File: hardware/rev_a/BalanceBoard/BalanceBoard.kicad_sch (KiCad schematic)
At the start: 49 parts, among them J1 47491-0001-TR425, J2 5103309-1, T00 TestPoints, T01 TestPoints, T02 TestPoints, T03 TestPoints, T04 TestPoints, T05 TestPoints, T06 TestPoints, T07 TestPoints, T10 TestPoints, T11 TestPoints, T12 TestPoints, T13 TestPoints, T14 TestPoints, T15 TestPoints, T16 TestPoints, T17 TestPoints, T21 TestPoints, T31 TestPoints, T32 TestPoints, T33 TestPoints, T40 TestPoints, T41 TestPoints, T42 TestPoints, T43 TestPoints, T44 TestPoints, T45 TestPoints, T46 TestPoints, T47 TestPoints, T48 TestPoints, T49 TestPoints, U1 C8051F850-A-GU, U2 FT232RL

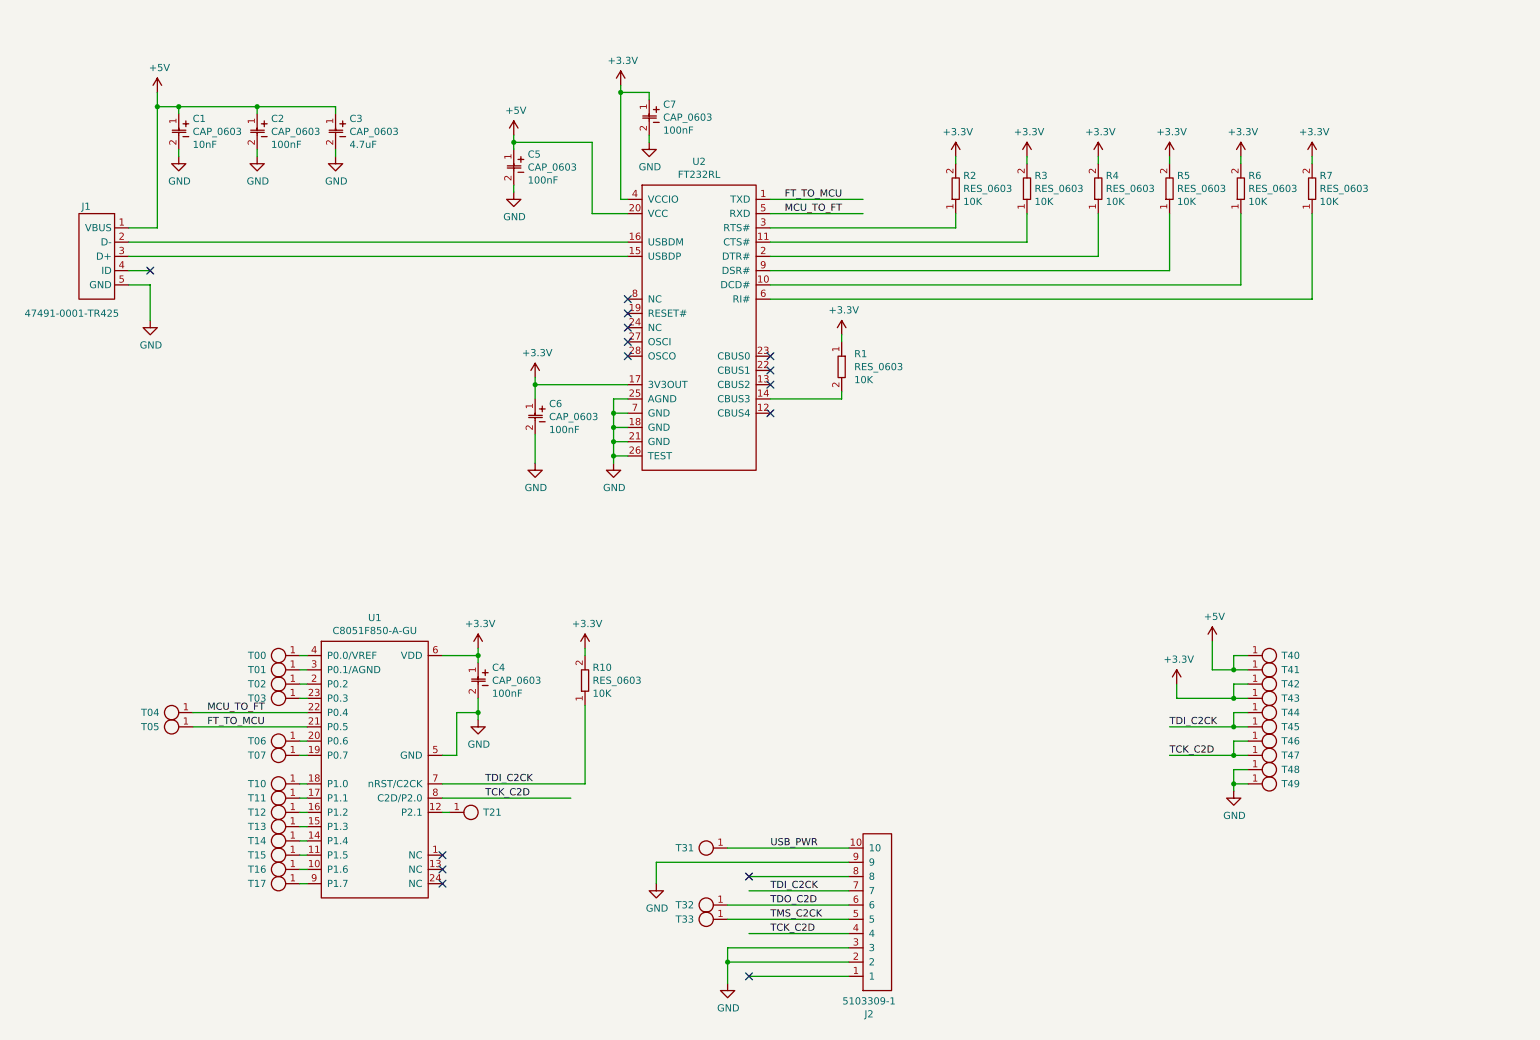
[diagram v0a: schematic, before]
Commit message: rev a fab out
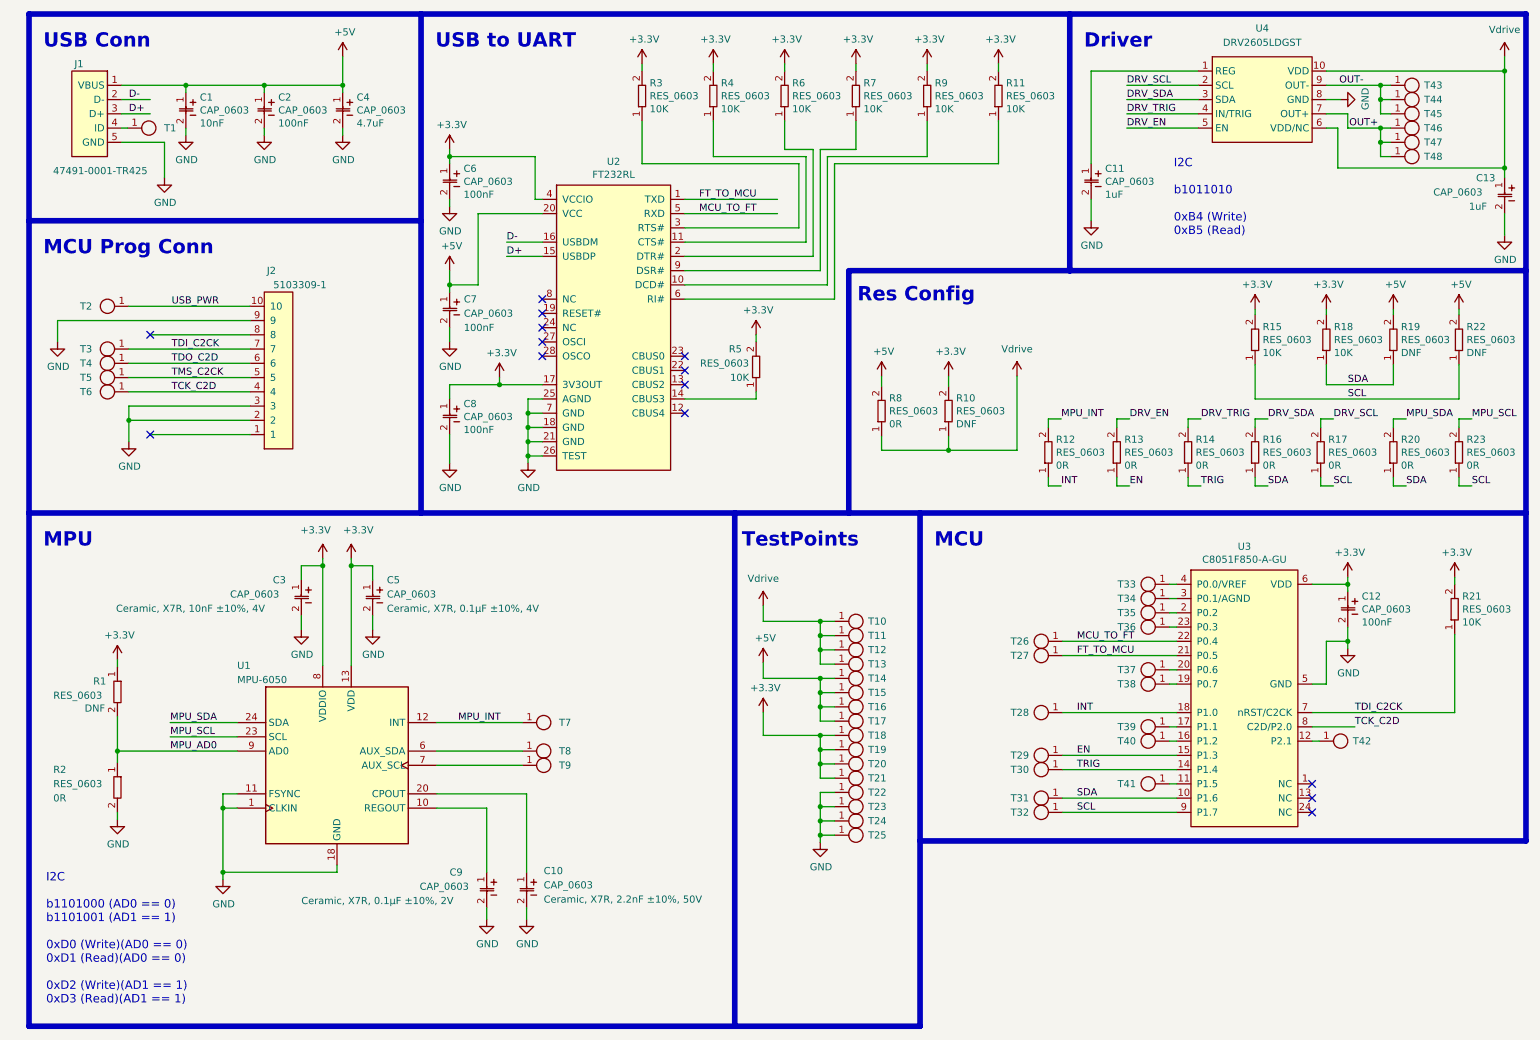
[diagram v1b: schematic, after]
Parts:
- added C10, C11, C13, C3, C5, C9: CAP_0603, receiver:0603, symbol BalanceBoard-rescue:CAP_0603-receiver
- added R1, R10, R12, R13, R14, R15, R16, R17, R18, R19, R2, R20, R22, R23, R8: RES_0603, receiver:0603, symbol BalanceBoard-rescue:RES_0603-receiver
- added T1, T10, T11, T12, T13, T16, T17, T19, T20, T22, T23, T43, T44, T45, T48, T7, T8, T9: TestPoints, receiver:TestPoint, symbol BalanceBoard-rescue:TestPoints-receiver
- added U1: MPU-6050, Sensor_Motion:InvenSense_QFN-24_4x4mm_P0.5mm, symbol Sensor_Motion:MPU-6050
- added U4: DRV2605LDGST, receiver:DRV2605LDGST, symbol BalanceBoard:DRV2605LDGST
- renumbered C4 to C12, C3 to C4, C7 to C6, C5 to C7, C6 to C8, R7 to R11, R10 to R21, R2 to R3, R3 to R4, R1 to R5, R4 to R6, R5 to R7, R6 to R9, T40 to T14, T41 to T15, T42 to T18, T31 to T2, T43 to T21, T48 to T24, T49 to T25, T04 to T26, T05 to T27, T10 to T28, T13 to T29, T44 to T3, T14 to T30, T16 to T31, T17 to T32, T00 to T33, T01 to T34, T02 to T35, T03 to T36, T06 to T37, T07 to T38, T11 to T39, T32 to T4, T12 to T40, T15 to T41, T21 to T42, T33 to T5, T45 to T6, U1 to U3
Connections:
- net +3V3: now also R5.2, C3.1, C5.1, R1.1, R10.2, R15.2, R18.2, T19.1, T20.1, U1.13 (VDD), U1.8 (VDDIO); no longer R5.1
- net +5V: now also R19.2, R22.2, R8.2, T16.1, T17.1
- net GND: now also C10.2, C11.2, C13.2, C3.2, C5.2, C9.2, R2.2, T22.1, T23.1, U1.1 (CLKIN), U1.11 (FSYNC), U1.18 (GND), U4.8 (GND)
- net TCK_C2D: now also T6.1; no longer T46.1, T47.1
- net TDI_C2CK: no longer T6.1
- net SDA: now reaches T31.1, U3.10 (P1.6)
- net SDA: now also R16.1, R18.1, R19.1, R20.1
- net TRIG: now reaches T30.1, U3.14 (P1.4)
- net TRIG: now also R14.1
- net EN: now reaches T29.1, U3.15 (P1.3)
- net EN: now also R13.1
- net INT: now reaches T28.1, U3.18 (P1.0)
- net INT: now also R12.1
- net SCL: now reaches T32.1, U3.9 (P1.7)
- net SCL: now also R15.1, R17.1, R22.1, R23.1
- net at U2.14 (CBUS3): now also R5.1; no longer R5.2
- net D+: now reaches J1.3 (D+), U2.15 (USBDP)
- net D-: now reaches J1.2 (D-), U2.16 (USBDM)
- net at J1.4 (ID): now also T1.1
- new net: C11.1, U4.1 (REG)
- new net: C9.1, U1.10 (REGOUT)
- new net: T8.1, U1.6 (AUX_SDA)
- new net: C10.1, U1.20 (CPOUT)
- new net: T9.1, U1.7 (AUX_SCL)
- new net DRV_EN: R13.2, U4.5 (EN)
- new net DRV_SCL: R17.2, U4.2 (SCL)
- new net DRV_SDA: R16.2, U4.3 (SDA)
- new net DRV_TRIG: R14.2, U4.4 (IN/TRIG)
- new net MPU_AD0: R1.2, R2.1, U1.9 (AD0)
- new net MPU_INT: R12.2, T7.1, U1.12 (INT)
- new net MPU_SCL: R23.2, U1.23 (SCL)
- new net MPU_SDA: R20.2, U1.24 (SDA)
- new net OUT+: T46.1, T47.1, T48.1, U4.7 (OUT+)
- new net OUT-: T43.1, T44.1, T45.1, U4.9 (OUT-)
- new net Vdrive: C13.1, R10.1, R8.1, T10.1, T11.1, T12.1, T13.1, U4.10 (VDD), U4.6 (VDD/NC)
- no-connect marks 15 -> 14
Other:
- note added: "Driver"
- note added: "I2C b1011010 0xB4 (Write) 0xB5 (Read)"
- note added: "I2C b1101000 (AD0 == 0) b1101001 (AD1 == 1) 0xD0 (Write)(AD0 == 0) 0xD1 (Read)(AD0 == 0) 0xD2 (Write)(AD1 == 1) 0xD3 (Read)(AD1 == 1)"
- note added: "MCU"
- note added: "MCU Prog Conn"
- note added: "MPU"
- note added: "Res Config"
- note added: "TestPoints"
- note added: "USB Conn"
- note added: "USB to UART"
- moved on the sheet: C1, C12, C2, C4, C6, C7, C8, R11, R21, R3, R4, R5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
